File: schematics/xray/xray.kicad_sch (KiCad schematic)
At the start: 103 parts, among them J1 USB_A, J2 USB_B_Micro, J3 USB_C_Receptacle_USB2.0, J4 USBASP, M1 VibroMotor, 3V, 8x2.7mm, Q1 IRF7413ZPbF, Q10 IRLML0030, Q11 IRLML0030, Q2 IRF7424PBF, Q3 IRLML0030, Q4 IRF7424PBF, Q5 IRLML0030, Q6 BC857, Q7 BC847, Q8 IRLML0030, Q9 IRLML0030, SW1 EC11W****, T1 Transformer_1P_1S, U1 IP5328P, U2 ATmega328P-A, U3 SN74LVC2T45DCUR, U4 SN74LVC2T45DCUR, U5 SN74LVC2T45DCUR, U6 Display_1.18inch_st7535, Y1 HC-49SM, 8MHz

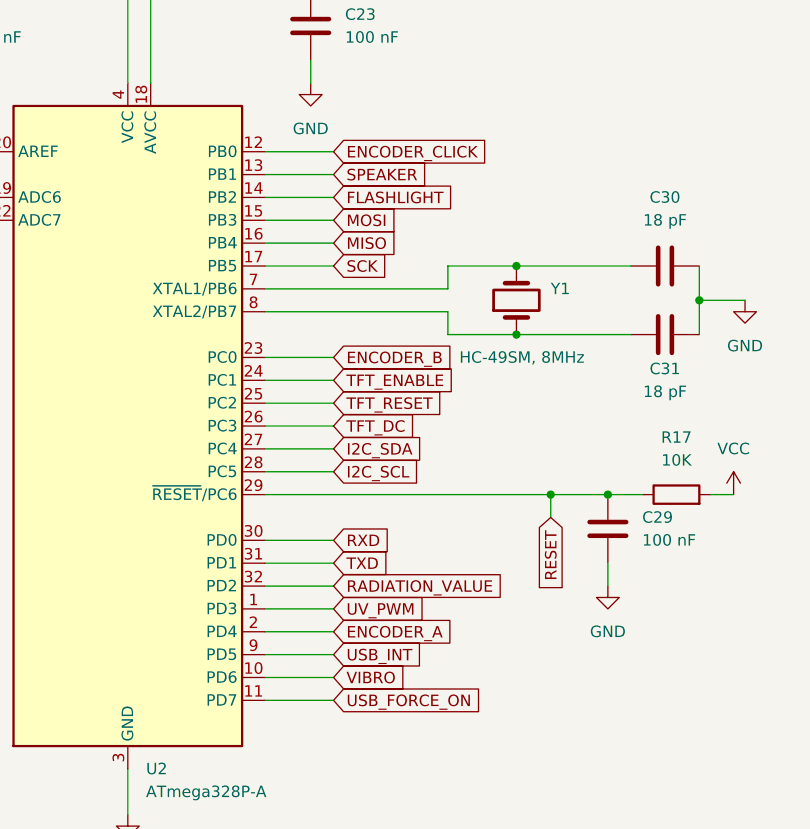
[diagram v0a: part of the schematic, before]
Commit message: debugging...
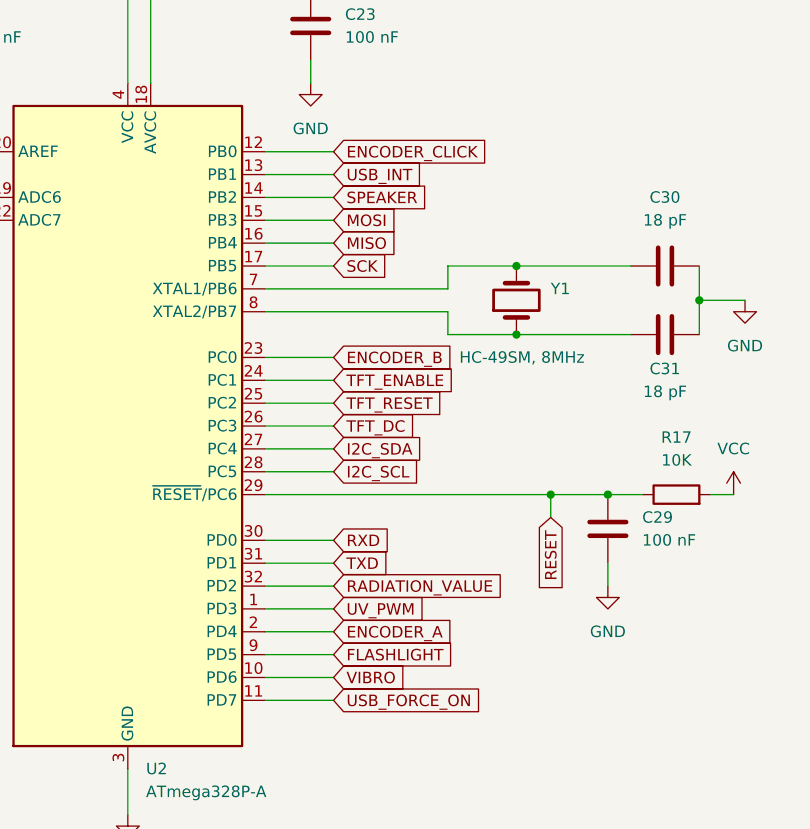
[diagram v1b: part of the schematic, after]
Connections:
- net FLASHLIGHT: now also U2.9 (PD5); no longer U2.14 (PB2)
- net SPEAKER: now also U2.14 (PB2); no longer U2.13 (PB1)
- net USB_INT: now also U2.13 (PB1); no longer U2.9 (PD5)
